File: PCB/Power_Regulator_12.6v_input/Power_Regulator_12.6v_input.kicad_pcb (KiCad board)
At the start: 2 copper layers, 90 x 90 mm, 65 parts, among them J1 SE2-30, J10 Conn_01x01_Pin, J12 Conn_01x01_Pin, J13 Conn_01x01_Pin, J2 Jack-DC, J3 Conn_01x05_Pin, J4 Conn_01x01_Pin, J5 Conn_01x01_Pin, J6 Conn_01x01_Pin, J7 Conn_01x01_Pin, J8 Conn_01x01_Pin, J9 Conn_01x01_Pin, SW1 SW_SPDT_321, U1 TLP3542, U2 TPS55340RTER, U3 TPS563203, U4 TPS54JA20RWWR

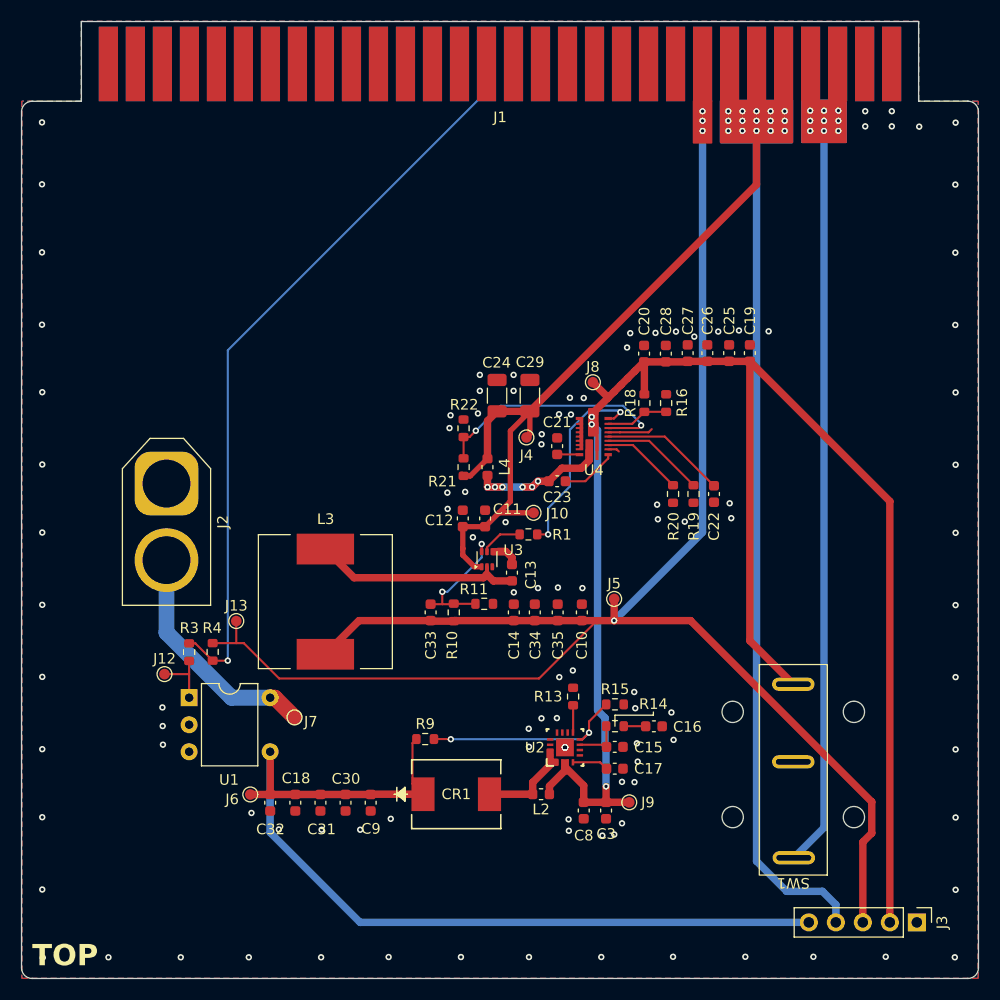
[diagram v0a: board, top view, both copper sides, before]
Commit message: edits from meeting
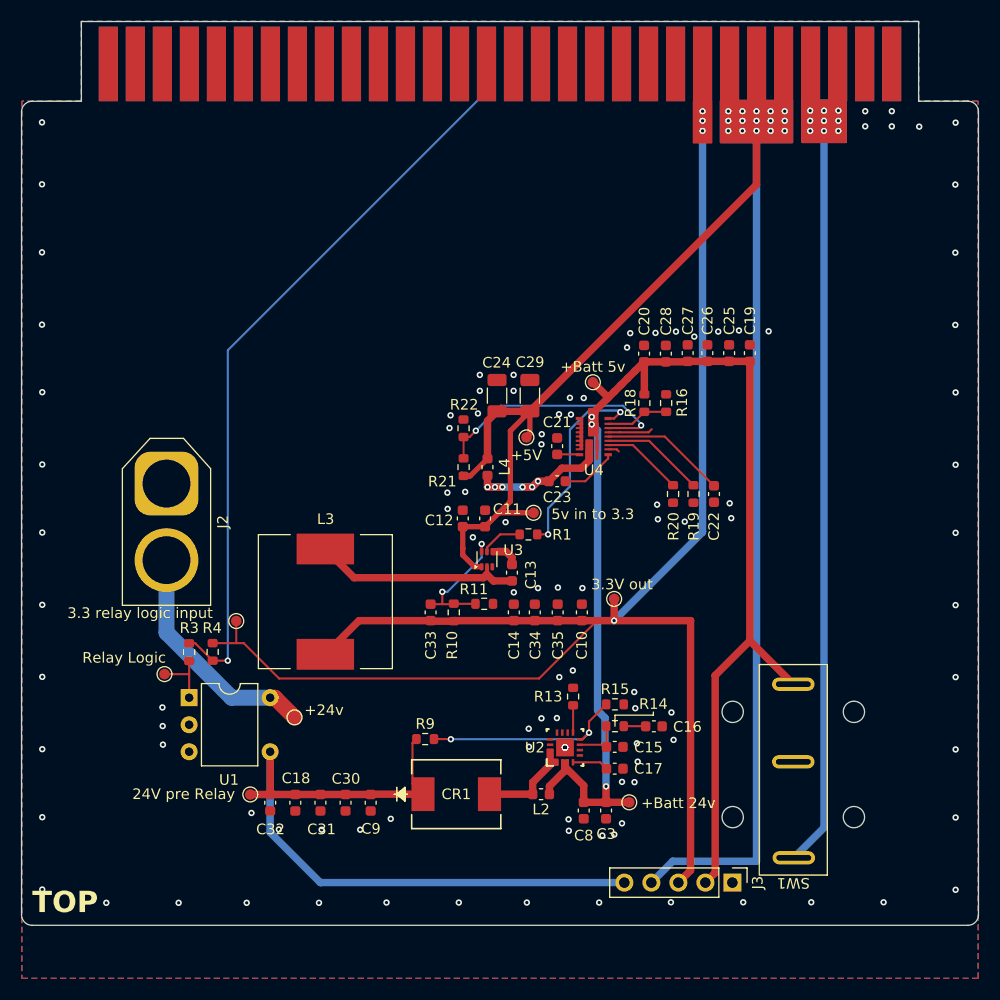
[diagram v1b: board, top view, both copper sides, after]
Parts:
- +Batt 24v: renamed from J9
- +Batt 5v: renamed from J8
- 24V pre Relay: renamed from J6
- 3.3 relay logic input: renamed from J13
- 3.3V out: renamed from J5
- 5v in to 3.3: renamed from J10
- Relay Logic: renamed from J12
- moved J3 17.7 mm to (161.1, 115.3)
- renumbered J7 to +24v, J4 to +5V
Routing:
- net +BATT: track 162.7 -> 128.9 mm
- net /24V_RAW: track 87.8 -> 68.9 mm
- net +3.3VA: track 171.2 -> 160.5 mm
- net GND: vias 111 -> 109
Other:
- board size 90 x 90 mm -> 90 x 85 mm
